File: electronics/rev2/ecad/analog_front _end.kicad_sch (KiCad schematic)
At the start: 23 parts, among them J3 Red Banana Plug, J4 Black Banana Plug, U10 MCP3561, U3 OPA4388IDR, U7 LM4030-2.5

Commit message: export
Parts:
- R1, R2, R42: Digikey Part # RMCF0805FT10K0CT-ND -> 311-10.0KCRCT-ND; Part # RMCF0805FT10K0 -> RC0805FR-0710KL
- R37: Unit Price (none) -> 0.13
- R39, R40, R41: Digikey Part # P10KDACT-ND -> YAG1763CT-ND; Part # ERA-6AEB103V -> RT0805BRD0710KL; Unit Price 0.32 -> 0.16
- R4: Digikey Part # (none) -> 311-10.0KCRCT-ND; Part # (none) -> RC0805FR-0710KL; Unit Price (none) -> 0.1
- R5: Digikey Part # (none) -> YAG1763CT-ND; Part # (none) -> RT0805BRD0710KL; Unit Price (none) -> 0.16
- S1: Digikey Part # (none) -> CWI359-ND; Part # (none) -> GF-161-0005; Unit Price (none) -> 1.97
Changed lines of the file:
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@@
 	(generator "eeschema")
 	(generator_version "8.0")
-	(paper "A4")
+	(paper "A")
 	(title_block
 		(title "Multimeter Analog Front End")
+		(date "2024-03-03")
+		(rev "1")
 	)
 	(junction
@@
 			)
 		)
+		(property "Digikey Part #" "YAG1763CT-ND"
+			(at 88.9 66.04 0)
+			(effects
+				(font
+					(size 1.27 1.27)
+				)
+				(hide yes)
+			)
+		)
+		(property "Part #" "RT0805BRD0710KL"
+			(at 88.9 66.04 0)
+			(effects
+				(font
+					(size 1.27 1.27)
+				)
+				(hide yes)
+			)
+		)
+		(property "Unit Price" "0.16"
+			(at 88.9 66.04 0)
+			(effects
+				(font
+					(size 1.27 1.27)
+				)
+				(hide yes)
+			)
+		)
 		(pin "1"
 		)
@@
 			)
 		)
-		(property "Digikey Part #" "RMCF0805FT10K0CT-ND"
+		(property "Digikey Part #" "311-10.0KCRCT-ND"
 			(at 201.93 147.32 0)
 			(effects
@@
 			)
 		)
-		(property "Part #" "RMCF0805FT10K0"
+		(property "Part #" "RC0805FR-0710KL"
 			(at 201.93 147.32 0)
 			(effects
@@
 			)
 		)
-		(property "Digikey Part #" "P10KDACT-ND"
+		(property "Digikey Part #" "YAG1763CT-ND"
 			(at 157.48 72.39 0)
 			(effects
@@
 			)
 		)
-		(property "Part #" "ERA-6AEB103V"
+		(property "Part #" "RT0805BRD0710KL"
 			(at 157.48 72.39 0)
 			(effects
@@
 			)
 		)
-		(property "Unit Price" "0.32"
+		(property "Unit Price" "0.16"
 			(at 157.48 72.39 0)
 			(effects
@@
 			)
 		)
-		(property "Digikey Part #" "RMCF0805FT10K0CT-ND"
+		(property "Digikey Part #" "311-10.0KCRCT-ND"
 			(at 213.36 39.37 0)
 			(effects
@@
 			)
 		)
-		(property "Part #" "RMCF0805FT10K0"
+		(property "Part #" "RC0805FR-0710KL"
 			(at 213.36 39.37 0)
 			(effects
@@
 			)
 		)
+		(property "Digikey Part #" "311-10.0KCRCT-ND"
+			(at 87.63 58.42 0)
+			(effects
+				(font
+					(size 1.27 1.27)
+				)
+				(hide yes)
+			)
+		)
+		(property "Part #" "RC0805FR-0710KL"
+			(at 87.63 58.42 0)
+			(effects
+				(font
+					(size 1.27 1.27)
+				)
+				(hide yes)
+			)
+		)
+		(property "Unit Price" "0.1"
+			(at 87.63 58.42 0)
+			(effects
+				(font
+					(size 1.27 1.27)
+				)
+				(hide yes)
+			)
+		)
 		(pin "2"
 		)
@@
 			)
 		)
-		(property "Digikey Part #" "RMCF0805FT10K0CT-ND"
+		(property "Digikey Part #" "311-10.0KCRCT-ND"
 			(at 201.93 137.16 0)
 			(effects
@@
 			)
 		)
-		(property "Part #" "RMCF0805FT10K0"
+		(property "Part #" "RC0805FR-0710KL"
 			(at 201.93 137.16 0)
 			(effects
@@
 			)
 		)
-		(property "Digikey Part #" "P10KDACT-ND"
+		(property "Digikey Part #" "YAG1763CT-ND"
 			(at 120.65 100.33 0)
 			(effects
@@
 			)
 		)
-		(property "Part #" "ERA-6AEB103V"
+		(property "Part #" "RT0805BRD0710KL"
 			(at 120.65 100.33 0)
 			(effects
@@
 			)
 		)
-		(property "Unit Price" "0.32"
+		(property "Unit Price" "0.16"
 			(at 120.65 100.33 0)
 			(effects
@@
 			)
 		)
+		(property "Digikey Part #" "CWI359-ND"
+			(at 107.95 49.53 0)
+			(effects
+				(font
+					(size 1.27 1.27)
+				)
+				(hide yes)
+			)
+		)
+		(property "Part #" "GF-161-0005"
+			(at 107.95 49.53 0)
+			(effects
+				(font
+					(size 1.27 1.27)
+				)
+				(hide yes)
+			)
+		)
+		(property "Unit Price" "1.97"
+			(at 107.95 49.53 0)
+			(effects
+				(font
+					(size 1.27 1.27)
+				)
+				(hide yes)
+			)
+		)
 		(pin "8"
 		)
@@
 			)
 		)
-		(property "Unit Price" ""
+		(property "Unit Price" "0.13"
 			(at 92.71 30.48 0)
 			(effects
@@
 			)
 		)
-		(property "Digikey Part #" "P10KDACT-ND"
+		(property "Digikey Part #" "YAG1763CT-ND"
 			(at 157.48 82.55 0)
 			(effects
@@
 			)
 		)
-		(property "Part #" "ERA-6AEB103V"
+		(property "Part #" "RT0805BRD0710KL"
 			(at 157.48 82.55 0)
 			(effects
@@
 			)
 		)
-		(property "Unit Price" "0.32"
+		(property "Unit Price" "0.16"
 			(at 157.48 82.55 0)
 			(effects

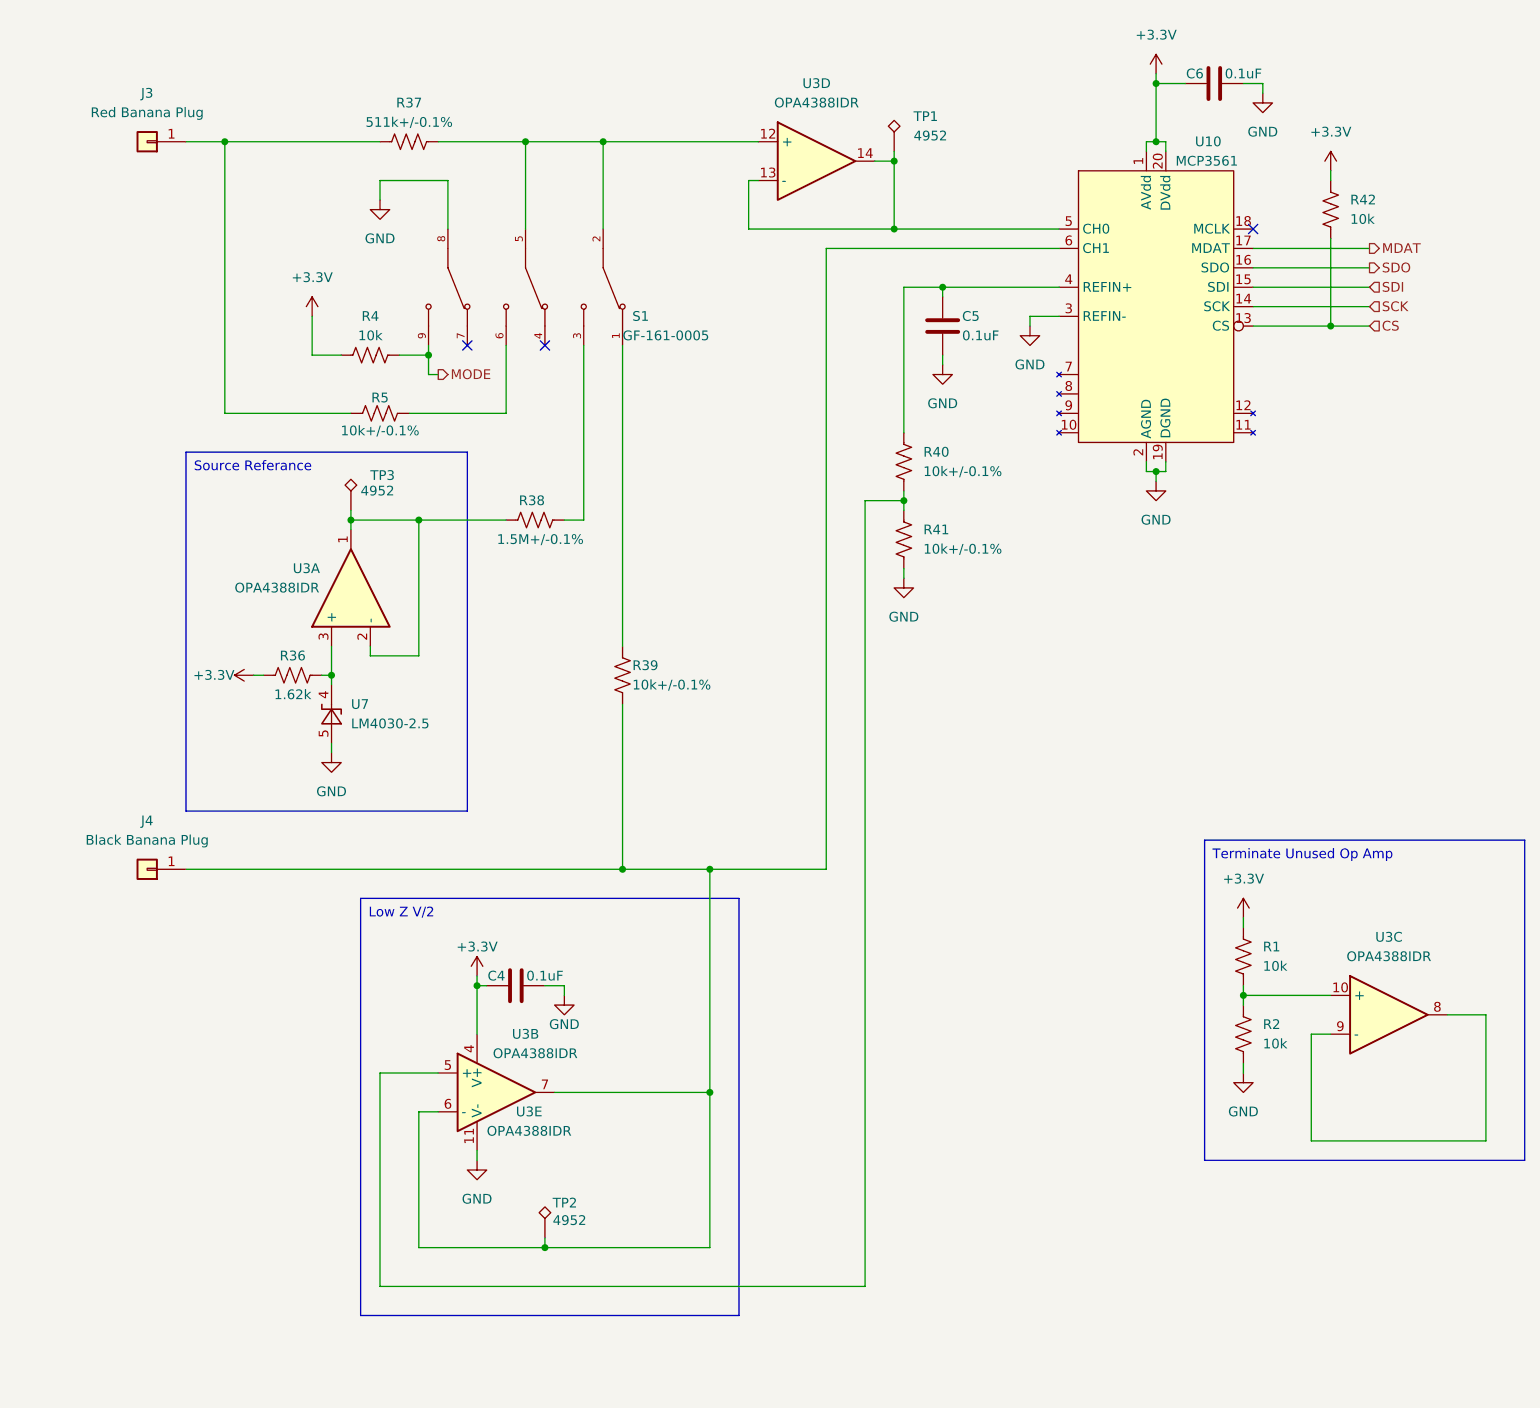
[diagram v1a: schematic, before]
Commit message: display doing stuff
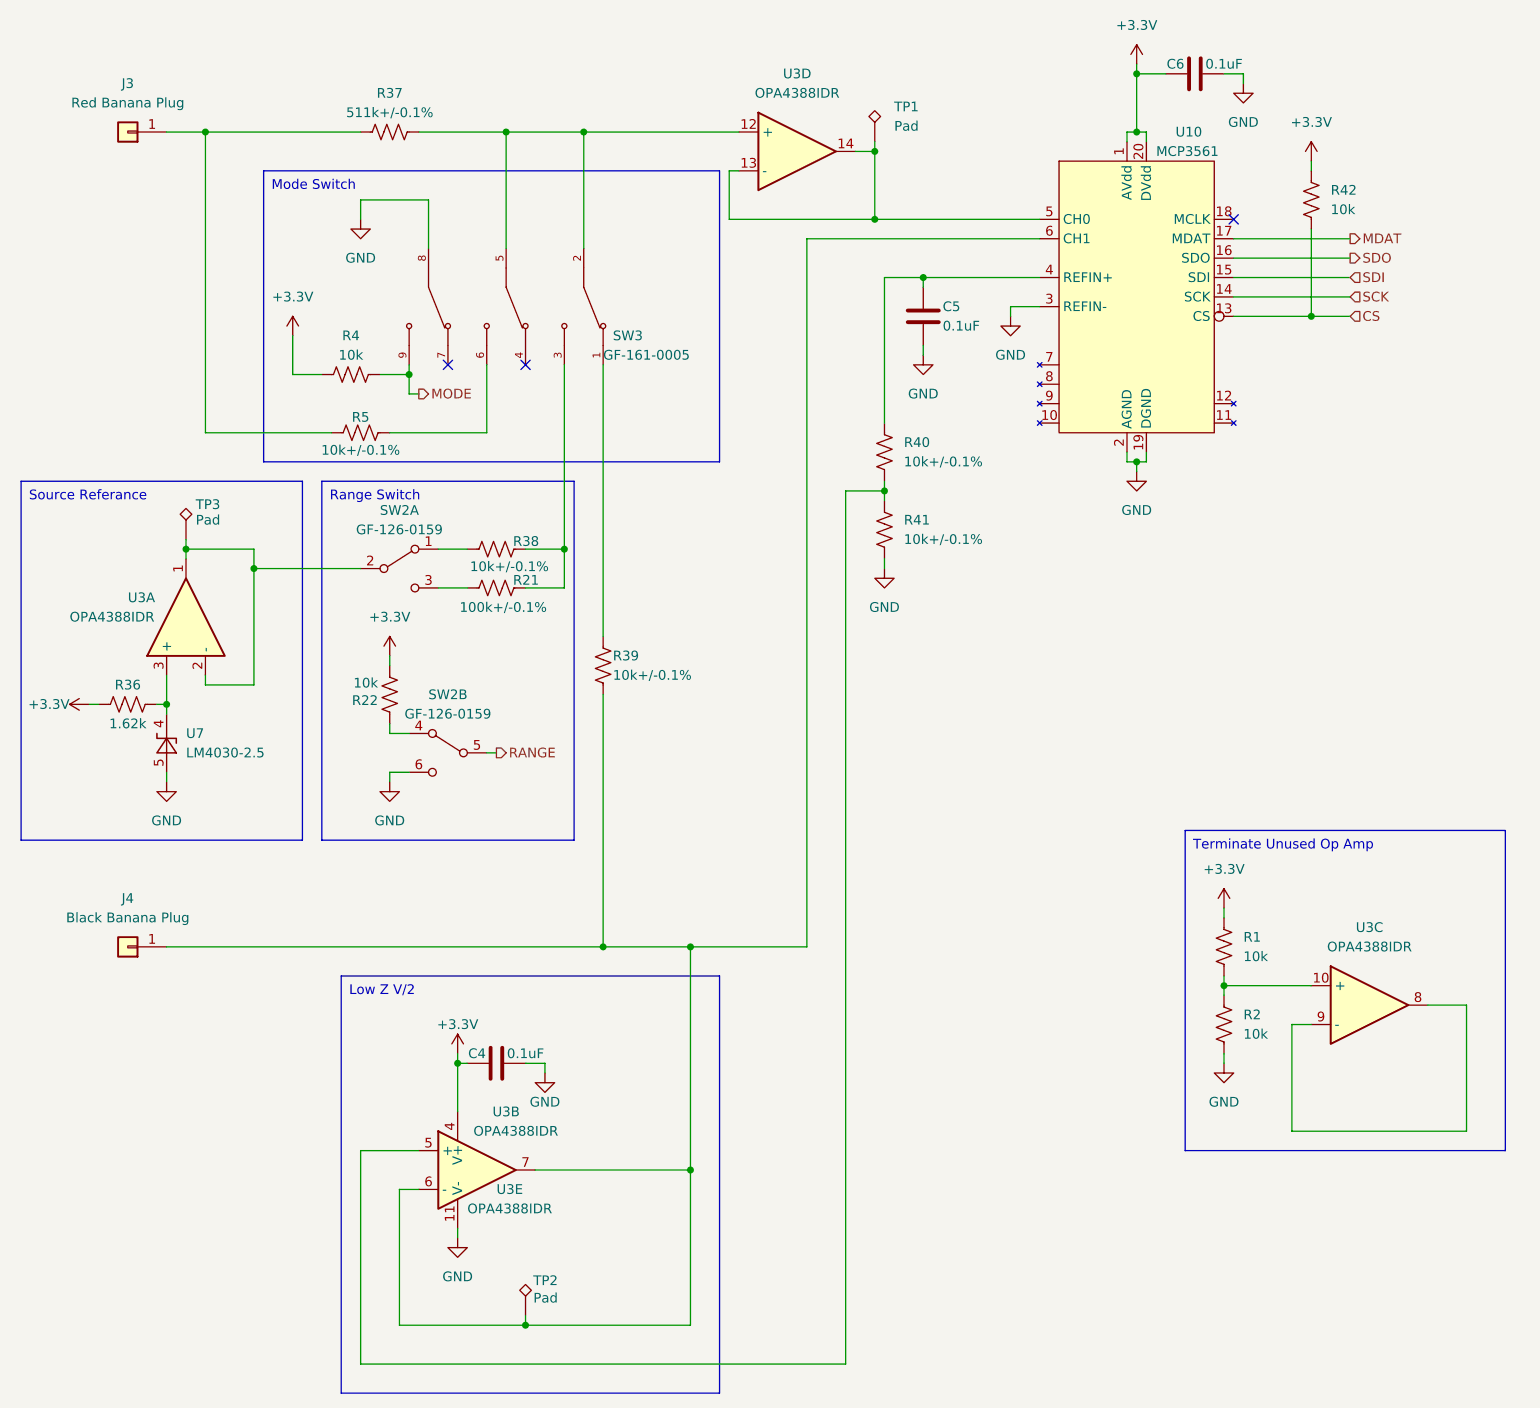
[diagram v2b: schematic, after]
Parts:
- added R21: 100k+/-0.1%, Resistor_SMD:R_0805_2012Metric_Pad1.20x1.40mm_HandSolder, symbol Device:R_US
- added R22: 10k, Resistor_SMD:R_0805_2012Metric_Pad1.20x1.40mm_HandSolder, symbol Device:R_US
- added SW2: GF-126-0159, Multimeter:SW_GF-126-0159, symbol Switch:SW_DPDT_x2
- R1, R2, R4, R42: Digikey Part # 311-10.0KCRCT-ND -> RMCF0805FT10K0CT-ND; Part # RC0805FR-0710KL -> RMCF0805FT10K0
- R38: value 1.5M+/-0.1% -> 10k+/-0.1%
- TP1, TP2, TP3: value 4952 -> Pad; Digikey Part # 36-4952-ND -> (none); Part # 4952 -> (none); Unit Price 0.26 -> (none)
- renumbered S1 to SW3
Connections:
- net +3.3V: now also R22.2
- net GND: now also SW2.6 (C)
- net at R38.2, SW3.3: now also R21.2
- net at TP3.1, U3.1, U3.2 (-): now also SW2.2 (B); no longer R38.1
- new net: R22.1, SW2.4 (A)
- new net: R38.1, SW2.1 (A)
- new net: R21.1, SW2.3 (C)
- new net RANGE: SW2.5 (B)
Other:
- moved on the sheet: C4, C5, C6, J3, J4, R1, R2, R36, R37, R38, R39, R4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

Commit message: ordered some stuff
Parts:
- R38: Digikey Part # 408-2025-1-ND -> P10KDACT-ND; Part # RG2012P-155-B-T5 -> ERA-6AEB103V; Unit Price 0.1 -> 0.13
- R39, R40, R41, R5: Digikey Part # YAG1763CT-ND -> P10KDACT-ND; Part # RT0805BRD0710KL -> ERA-6AEB103V; Unit Price 0.16 -> 0.13
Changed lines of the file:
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@@
 			)
 		)
-		(property "Digikey Part #" "YAG1763CT-ND"
+		(property "Digikey Part #" "P10KDACT-ND"
 			(at 86.36 68.58 0)
 			(effects
@@
 			)
 		)
-		(property "Part #" "RT0805BRD0710KL"
+		(property "Part #" "ERA-6AEB103V"
 			(at 86.36 68.58 0)
 			(effects
@@
 			)
 		)
-		(property "Unit Price" "0.16"
+		(property "Unit Price" "0.13"
 			(at 86.36 68.58 0)
 			(effects
@@
 			)
 		)
-		(property "Digikey Part #" "YAG1763CT-ND"
+		(property "Digikey Part #" "P10KDACT-ND"
 			(at 154.94 71.12 0)
 			(effects
@@
 			)
 		)
-		(property "Part #" "RT0805BRD0710KL"
+		(property "Part #" "ERA-6AEB103V"
 			(at 154.94 71.12 0)
 			(effects
@@
 			)
 		)
-		(property "Unit Price" "0.16"
+		(property "Unit Price" "0.13"
 			(at 154.94 71.12 0)
 			(effects
@@
 			)
 		)
-		(property "Digikey Part #" "YAG1763CT-ND"
+		(property "Digikey Part #" "P10KDACT-ND"
 			(at 118.11 99.06 0)
 			(effects
@@
 			)
 		)
-		(property "Part #" "RT0805BRD0710KL"
+		(property "Part #" "ERA-6AEB103V"
 			(at 118.11 99.06 0)
 			(effects
@@
 			)
 		)
-		(property "Unit Price" "0.16"
+		(property "Unit Price" "0.13"
 			(at 118.11 99.06 0)
 			(effects
@@
 			)
 		)
-		(property "Digikey Part #" "408-2025-1-ND"
+		(property "Digikey Part #" "P10KDACT-ND"
 			(at 104.14 83.82 0)
 			(effects
@@
 			)
 		)
-		(property "Part #" "RG2012P-155-B-T5"
+		(property "Part #" "ERA-6AEB103V"
 			(at 104.14 83.82 0)
 			(effects
@@
 			)
 		)
-		(property "Unit Price" "0.1"
+		(property "Unit Price" "0.13"
 			(at 104.14 83.82 0)
 			(effects
@@
 			)
 		)
-		(property "Digikey Part #" "YAG1763CT-ND"
+		(property "Digikey Part #" "P10KDACT-ND"
 			(at 154.94 81.28 0)
 			(effects
@@
 			)
 		)
-		(property "Part #" "RT0805BRD0710KL"
+		(property "Part #" "ERA-6AEB103V"
 			(at 154.94 81.28 0)
 			(effects
@@
 			)
 		)
-		(property "Unit Price" "0.16"
+		(property "Unit Price" "0.13"
 			(at 154.94 81.28 0)
 			(effects
